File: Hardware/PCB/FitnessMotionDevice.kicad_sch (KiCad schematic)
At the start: 51 parts, among them J1 USB_C_Receptacle_USB2.0_16P, J2 Conn_01x02_MountingPin, J3 Conn_01x04, J4 Conn_01x04, U1 nRF52840, U2 BQ24074RGT, U3 USBLC6-2SC6, U7 LSM6DSVTR, Y2 Crystal_GND23

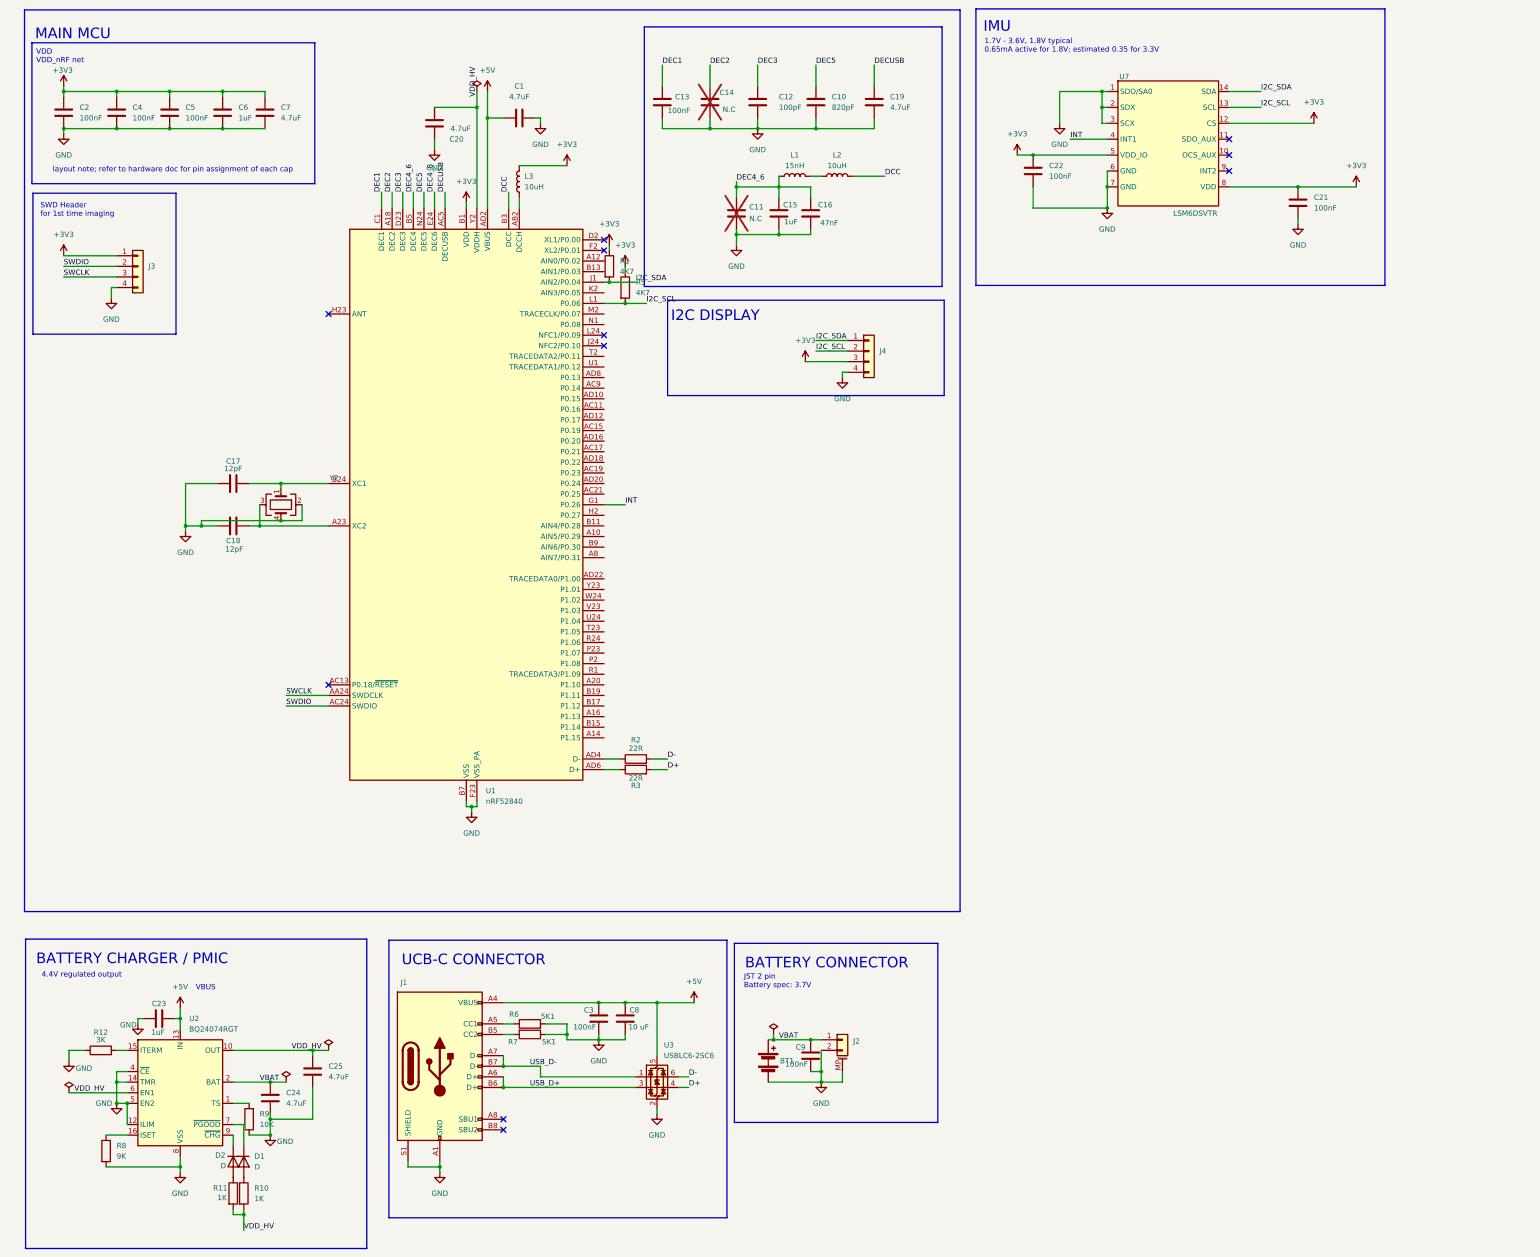
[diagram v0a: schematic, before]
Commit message: added readme
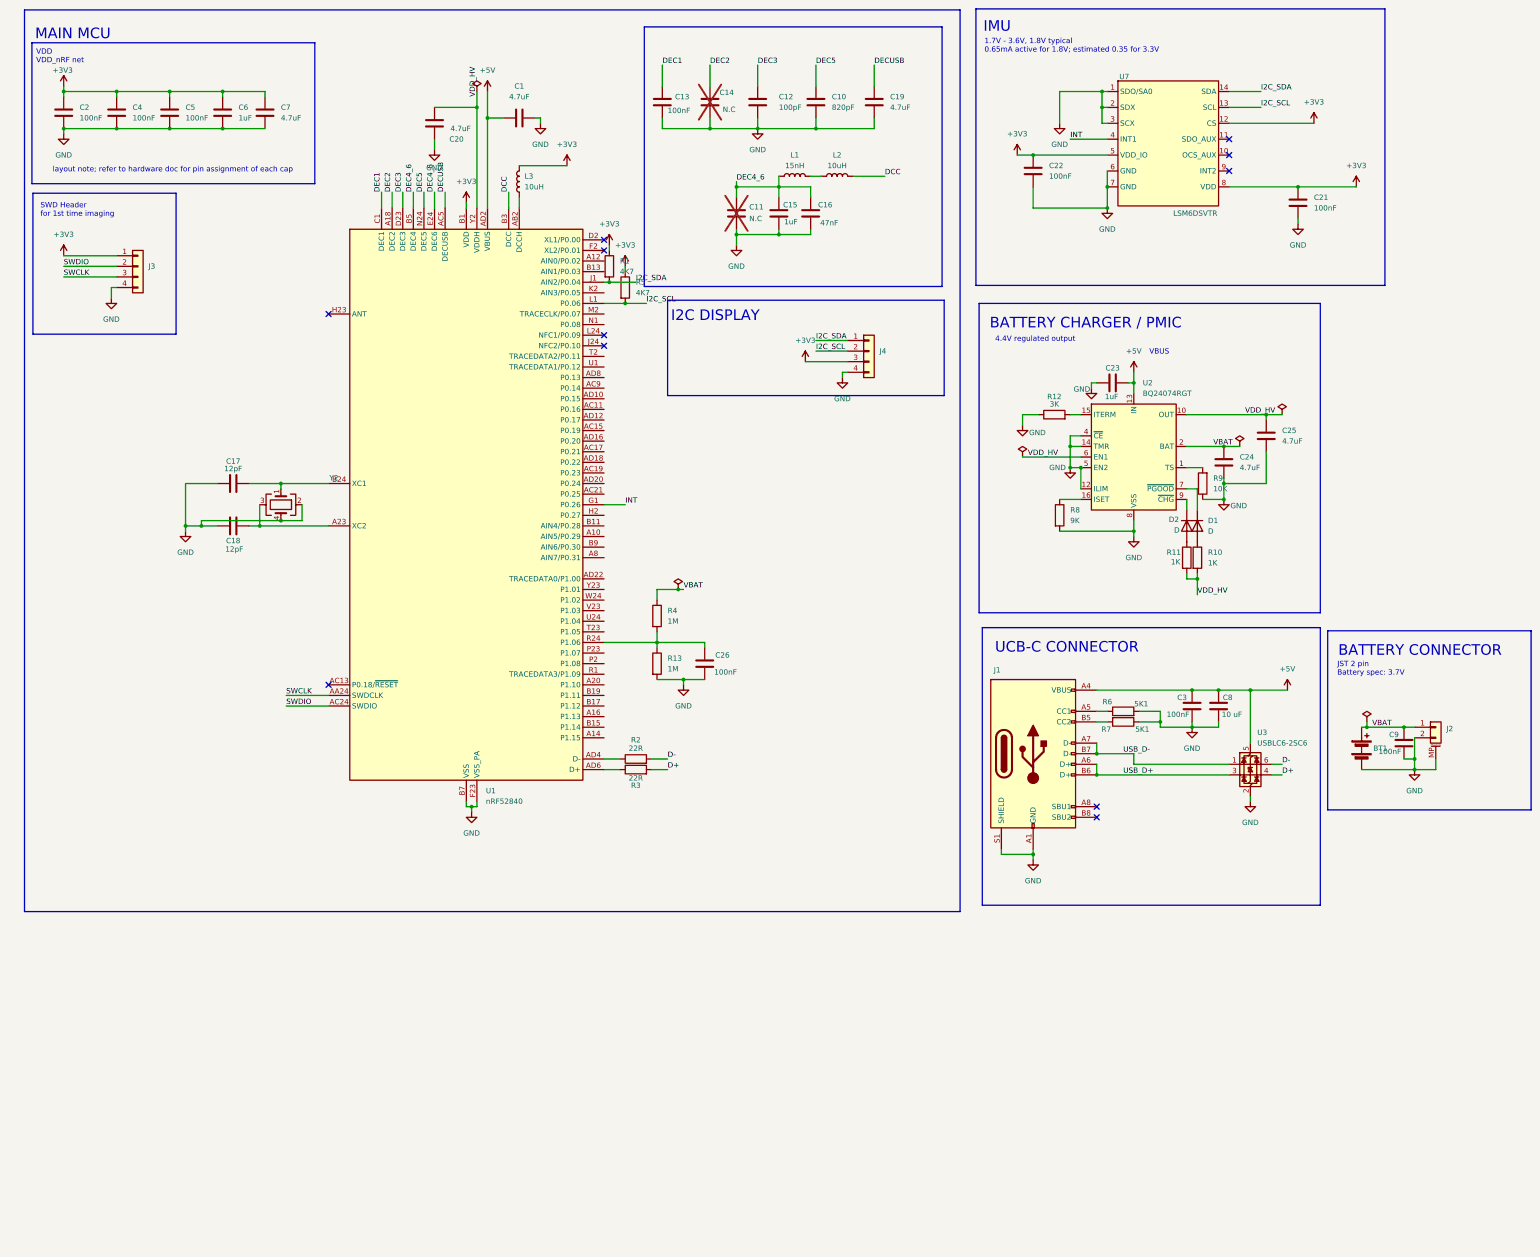
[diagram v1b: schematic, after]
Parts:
- added C26: 100nF, Capacitor_SMD:C_0603_1608Metric, symbol Device:C
- added R13, R4: 1M, Resistor_SMD:R_0402_1005Metric, symbol Device:R
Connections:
- net GND: now also C26.1, R13.2
- net VBAT: now also R4.1
- net at U1.R24 (P1.06): now also C26.2, R13.1, R4.2
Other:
- moved on the sheet: BT1, C23, C24, C25, C3, C8, C9, D1, D2, J1, J2, R10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
